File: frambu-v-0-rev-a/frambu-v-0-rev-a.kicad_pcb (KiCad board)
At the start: 2 copper layers, 40 x 55 mm, 31 parts, among them J1 USB_C_Receptacle_USB2.0_16P, J2 pico_pines_1-20, J3 SWD, J5 pico_pines_40-21, SW1 PTS 636, U1 W25Q128JVS, U2 RP2040, U3 AMS1117-3.3, Y1 12MHz

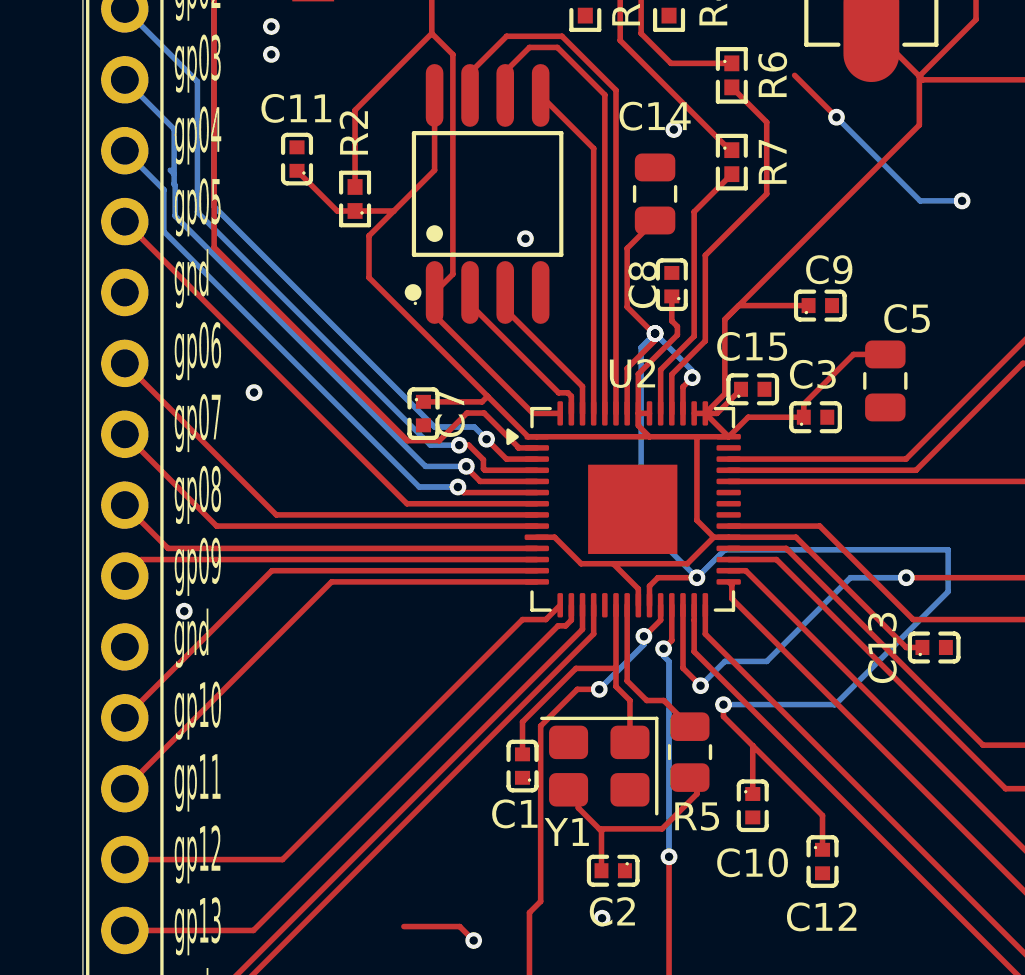
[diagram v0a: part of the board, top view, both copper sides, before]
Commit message: agreagr
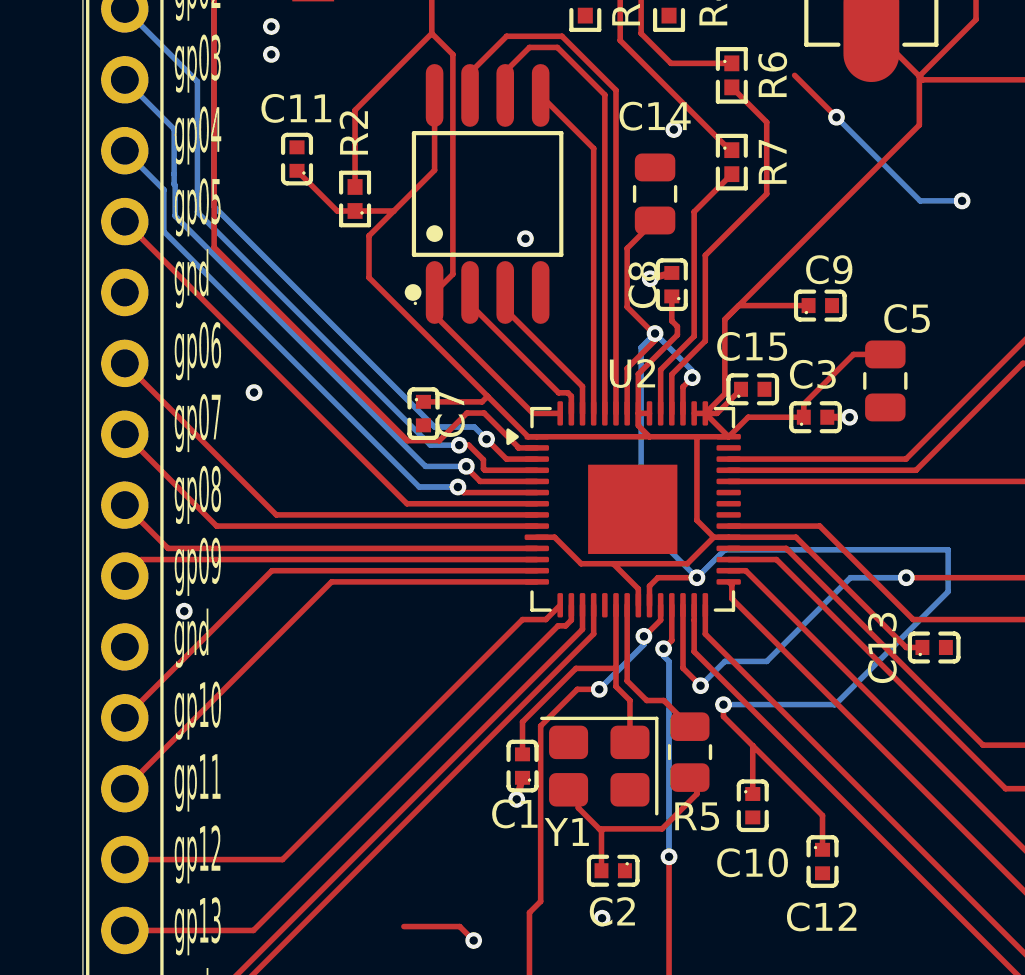
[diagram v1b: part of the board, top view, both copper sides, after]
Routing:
- net GND: track 29.0 -> 31.4 mm, vias 19 -> 22
- net +1V1: vias 5 -> 4
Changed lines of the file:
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@@
+	)
+	(segment
+		(start 41.1 41.08)
+		(end 40.32726 41.287055)
+		(width 0.25)
+		(layer "F.Cu")
+		(net "GND")
 	)
 	(segment
@@
 	)
 	(segment
+		(start 35.75 59.17)
+		(end 35.542945 59.94274)
+		(width 0.25)
+		(layer "F.Cu")
+		(net "GND")
+	)
+	(segment
 		(start 45.5 34)
 		(end 47 35.5)
@@
 	)
 	(segment
+		(start 46.67 46.25)
+		(end 47.47 46.25)
+		(width 0.25)
+		(layer "F.Cu")
+		(net "GND")
+	)
+	(segment
 		(start 43.25 28.045)
 		(end 43.405 28.045)
@@
 	)
 	(via
+		(at 40.32726 41.287055)
+		(size 0.6)
+		(drill 0.3)
+		(layers "F.Cu" "B.Cu")
+		(net "GND")
+	)
+	(via
 		(at 56.296359 42.617429)
 		(size 0.6)
@@
 	)
 	(via
+		(at 47.47 46.25)
+		(size 0.6)
+		(drill 0.3)
+		(layers "F.Cu" "B.Cu")
+		(net "GND")
+	)
+	(via
 		(at 26.129409 45.365859)
 		(size 0.6)
@@
 	(via
 		(at 23.629407 53.2005)
+		(size 0.6)
+		(drill 0.3)
+		(layers "F.Cu" "B.Cu")
+		(net "GND")
+	)
+	(via
+		(at 35.542945 59.94274)
 		(size 0.6)
 		(drill 0.3)
@@
 	)
 	(via
-		(at 40.5 43.25)
-		(size 0.6)
-		(drill 0.3)
-		(layers "F.Cu" "B.Cu")
-		(net "+1V1")
-	)
-	(via
 		(at 41.832108 44.832108)
 		(size 0.6)
@@
 		(width 0.2)
 		(layer "B.Cu")
-		(net "/GPIO03")
-	)
-	(segment
-		(start 23.263766 37.536234)
-		(end 23.127533 37.4)
-		(width 0.2)
-		(layer "B.Cu")
